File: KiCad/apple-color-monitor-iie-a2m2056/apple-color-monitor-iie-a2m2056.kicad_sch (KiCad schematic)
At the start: 467 parts, among them CN14 Conn_01x04_Pin, CN16 Conn_01x01_Pin, CN20 Conn_01x06_Pin, CN20_plug1 Conn_01x06, CN4 Conn_01x07_Pin, CN4_FRONT1 CN, CN5 Text/Gfx, CN5_FRONT1 Conn_01x02_Socket, CN8 Conn_01x02_Pin, CN9 Conn_01x02_Pin, IC102 CD4053B, J101 Jumper_2_Bridged, J102 Jumper_2_Bridged, J103 Jumper_2_Bridged, J104 Jumper_2_Bridged, J106 Jumper_2_Bridged, J107 Jumper_2_Bridged, J108 Jumper_2_Bridged, J109 Jumper_2_Bridged, J110 Jumper_2_Bridged, J111 Jumper_2_Bridged, J112 Jumper_2_Bridged, J113 Jumper_2_Bridged, J114 Jumper_2_Bridged, J201 Jumper_2_Bridged, J202 Jumper_2_Bridged, J203 Jumper_2_Bridged, J204 Jumper_2_Bridged, J205 Jumper_2_Bridged, J206 Jumper_2_Bridged, J207 Jumper_2_Bridged, J302 Jumper_2_Bridged, J304 Jumper_2_Bridged, J306 Jumper_2_Bridged, J308 Jumper_2_Bridged, J401 Jumper_2_Bridged, J402 Jumper_2_Bridged, J502 Jumper_2_Bridged, J603 Jumper_2_Bridged, J604 Jumper_2_Bridged, J801 Jumper_2_Bridged, J802 Jumper_2_Bridged, J803 Jumper_2_Bridged, J804 Jumper_2_Bridged, J805 Jumper_2_Bridged, J806 Jumper_2_Bridged, J871 Jumper_2_Bridged, J901 Jumper_2_Bridged, P1_P2 IN PUT, P3 Conn_01x01_Pin, P701 VIDEO IN, Q101 C945, Q102 A733, Q103 A733, Q104 C945, Q105 A733, Q111 A642, Q114 C945, Q201 C1507, Q202 D1398, Q501 A709, Q502 C1008, Q503 C3042, Q504 A709, Q801 C945, Q802 C945, Q803 C945, Q804 A733, Q805 A733, Q806 A733, Q807 A733, Q808 A733, Q809 A733, Q901 C1507, Q902 C1507, Q903 C1507, Q904 C2330, Q905 C2330, Q906 C2330, SW1 SW_SPST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

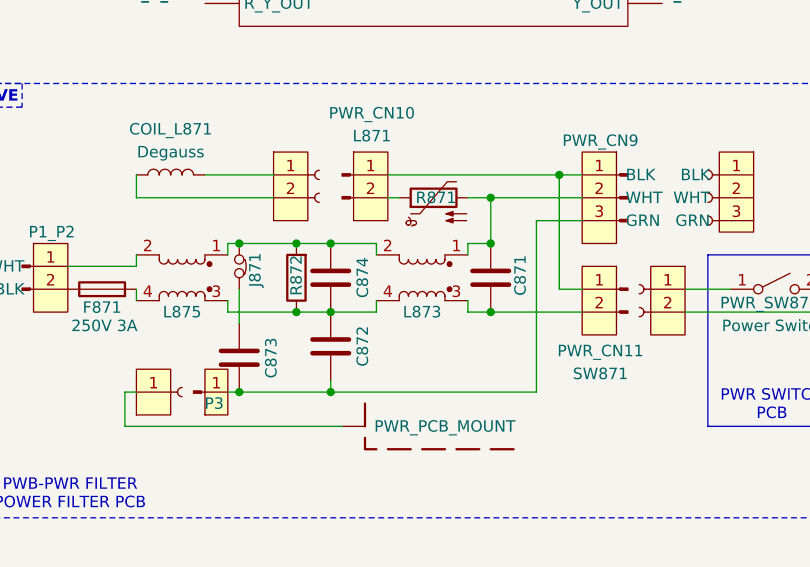
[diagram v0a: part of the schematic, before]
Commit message: checkpoint
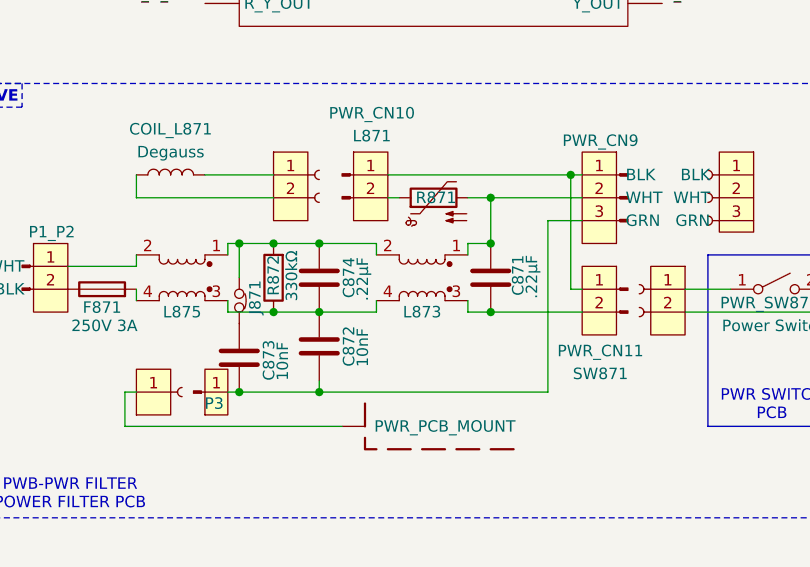
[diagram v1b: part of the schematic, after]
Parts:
- C871, C874: value C -> .22µF
- C872, C873: value C -> 10nF
- R872: value R -> 330kΩ
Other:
- moved on the sheet: C872, C874, J871, R872
